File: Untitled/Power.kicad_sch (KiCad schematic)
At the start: 25 parts, among them J2 USB4125-GF-A-0190, U2 INA180A1, U3 SPX3819M5-L-3-3, U4 SPX3819M5-L-3-3, U5 TPS7A0522PDBZT

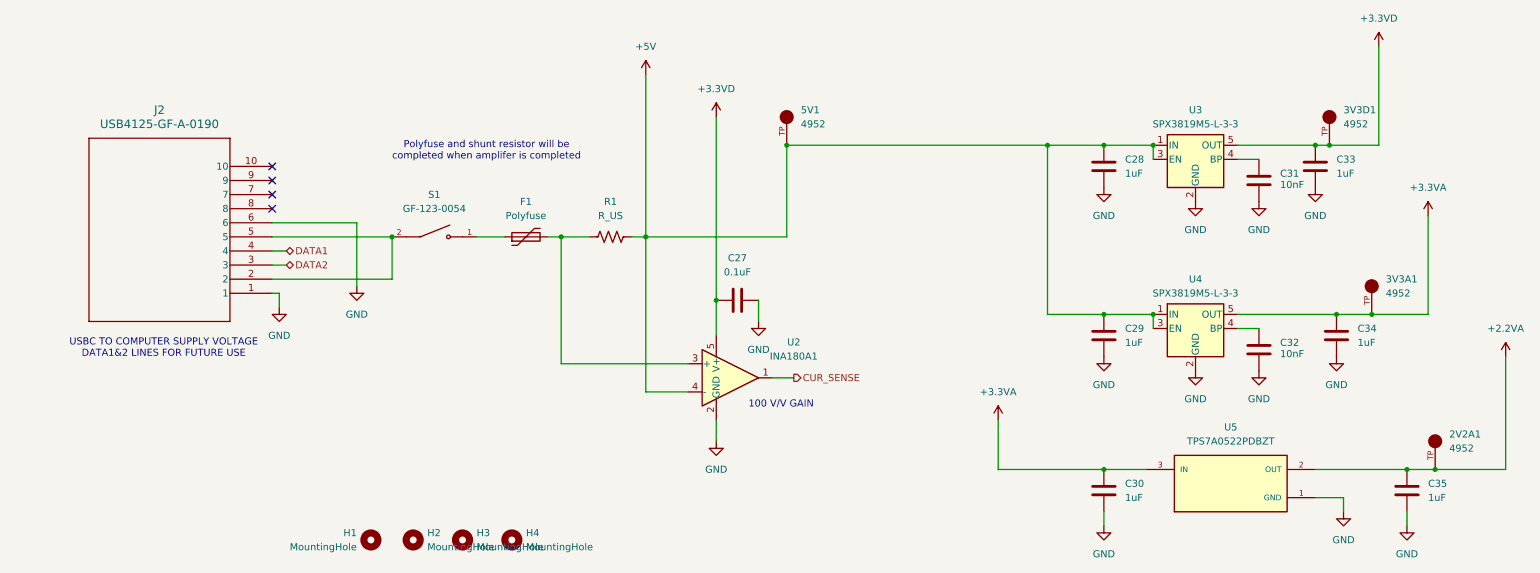
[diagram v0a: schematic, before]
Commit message: fixed board
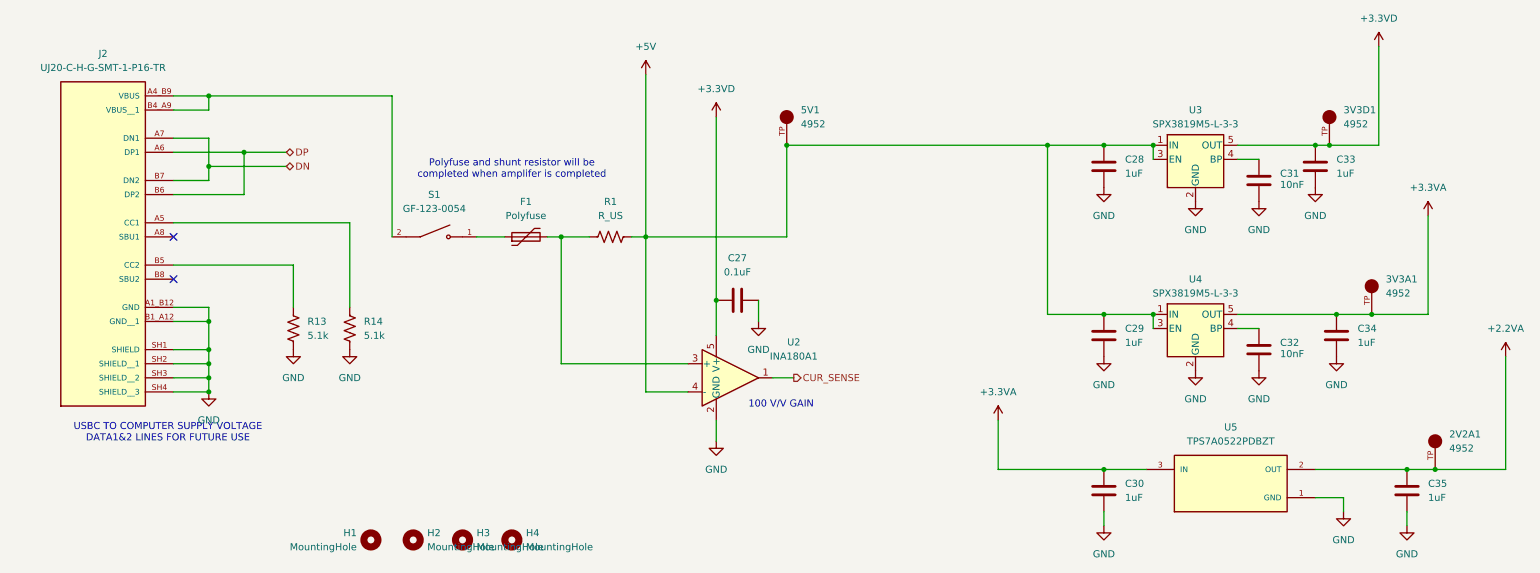
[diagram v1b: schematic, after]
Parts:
- removed J2: USB4125-GF-A-0190, USB-c:CONN6_125-GF-A-0190_GCT, symbol USB-c:USB4125-GF-A-0190
- added J2: UJ20-C-H-G-SMT-1-P16-TR, USB-c:SAMESKY_UJ20-C-H-G-SMT-1-P16-TR, symbol UJ20-C-H-G-SMT-1-P16-TR:UJ20-C-H-G-SMT-1-P16-TR
- added R13, R14: 5.1k, Resistor_SMD:R_0805_2012Metric_Pad1.20x1.40mm_HandSolder, symbol Device:R_US
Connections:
- net GND: now also J2.A1_B12 (GND), J2.B1_A12 (GND__1), J2.SH1 (SHIELD), J2.SH2 (SHIELD__1), J2.SH3 (SHIELD__2), J2.SH4 (SHIELD__3), R13.2, R14.2
- net at S1.2: now also J2.A4_B9 (VBUS), J2.B4_A9 (VBUS__1)
- new net: J2.A5 (CC1), R14.1
- new net: J2.B5 (CC2), R13.1
- new net DN: J2.A7 (DN1), J2.B7 (DN2)
- new net DP: J2.A6 (DP1), J2.B6 (DP2)
- no-connect marks 4 -> 2
